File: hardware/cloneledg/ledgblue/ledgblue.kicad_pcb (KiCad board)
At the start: 2 copper layers, 62.4 x 46.9 mm, 61 parts, among them J1 USB_OTG, P1 DEBUG, P2 DEBUG, P3 YL035MY2, P4 YL035MY2_TS_WURTH, SW1 WURTH 436353045816, SW2 SW-PB, U1 LD39020_3.0V, U2 STMPS2151TTR, U3 ST31G480, U4 STM32L476RCT6, U5 AMS_AS3921, U6 STNS01PUR, U7 SPBTLE-RF, U8 STLA02PUR, Y1 8 MHz

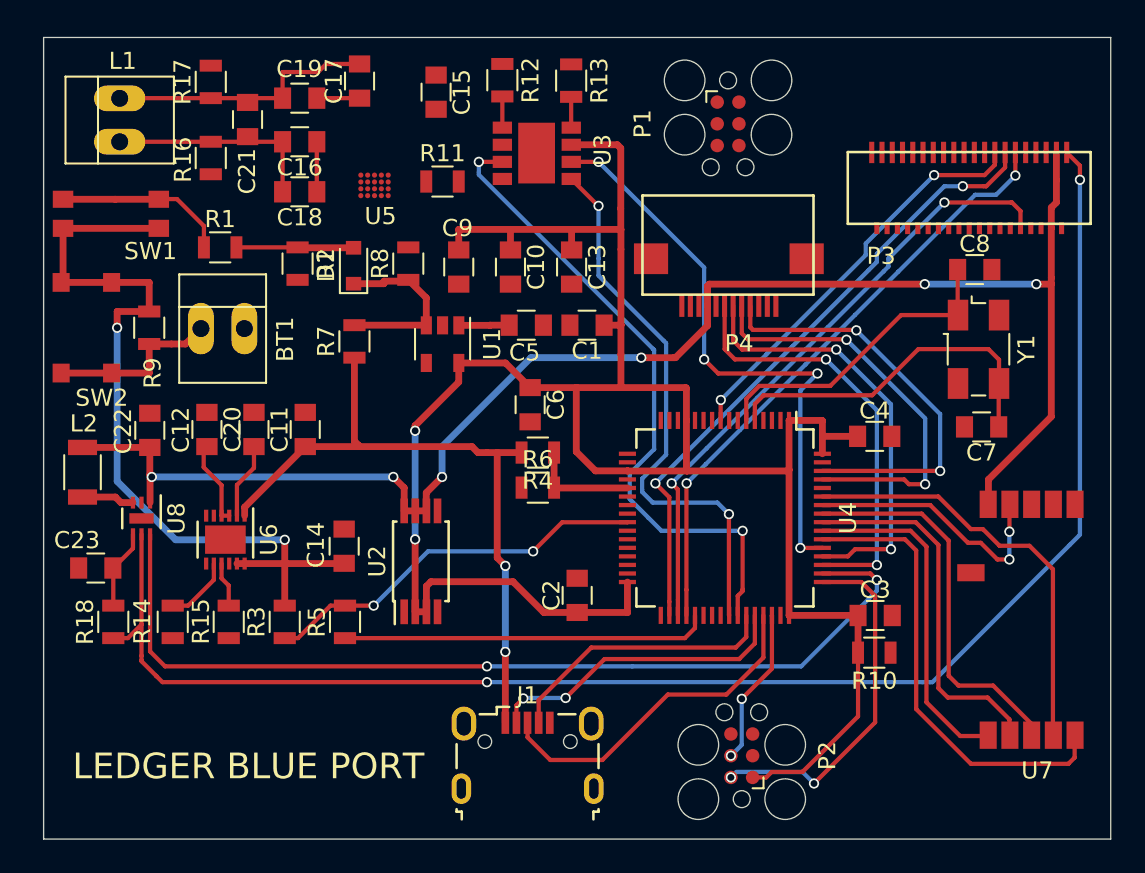
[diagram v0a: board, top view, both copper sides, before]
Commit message: Ledger Blue port finished
Everything is connected!
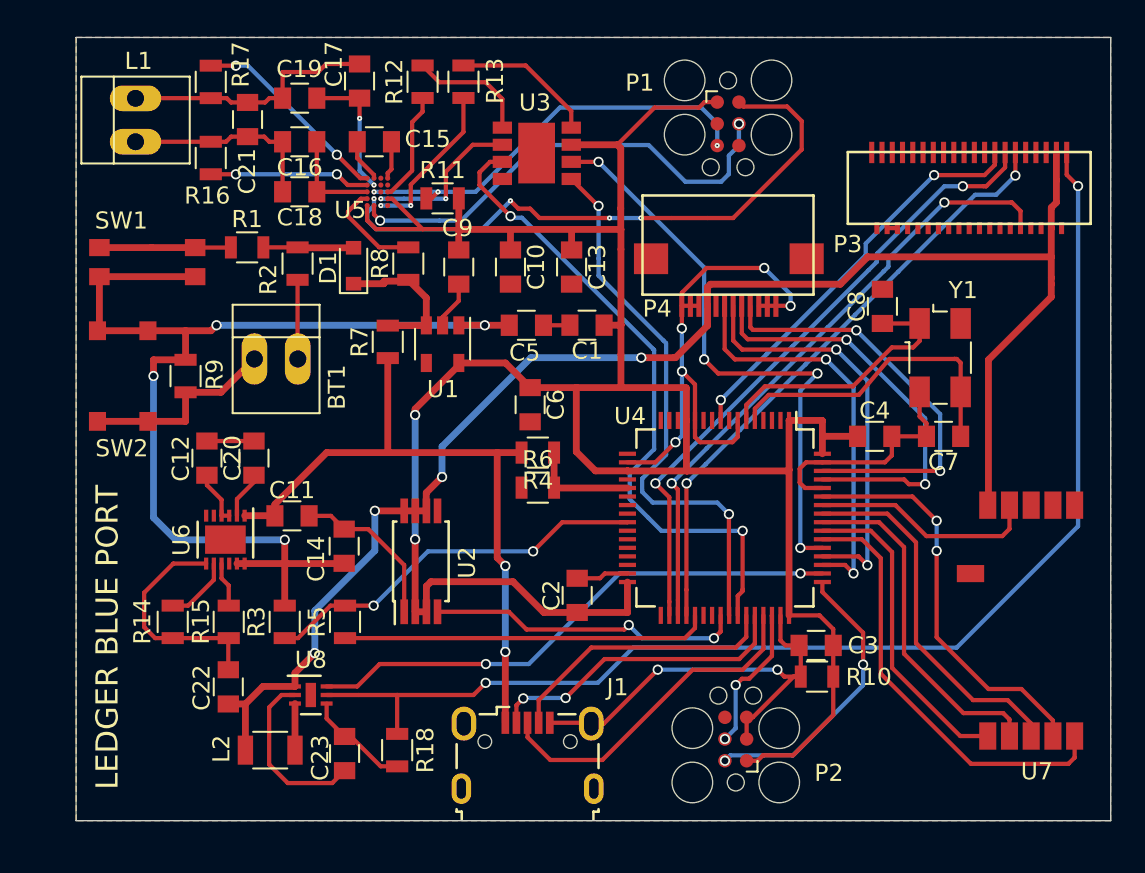
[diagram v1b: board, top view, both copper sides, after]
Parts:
- moved L2 19.6 mm to (39.0, 179.3), turned to 180 degrees
- moved R18 18.2 mm to (46.5, 179.3), turned to 270 degrees
- moved C23 18.2 mm to (43.4, 179.5), turned to 270 degrees
- moved C22 15.7 mm to (36.6, 175.6)
- moved U8 14.3 mm to (41.4, 176.1), turned to 0 degrees
- moved R13 6.30 mm to (50.4, 140.2), turned to 90 degrees
- moved C8 5.81 mm to (74.8, 153.3), turned to 90 degrees
- moved C11 5.11 mm to (40.3, 165.6), turned to 0 degrees
- moved R12 4.67 mm to (48.0, 140.2), turned to 90 degrees
- moved C15 4.63 mm to (45.1, 143.7), turned to 0 degrees
- moved C3 3.87 mm to (71.0, 173.2), turned to 180 degrees
- moved R10 3.63 mm to (71.0, 175.0), turned to 0 degrees
- moved BT1 3.59 mm to (38.1, 156.4)
- moved R9 3.54 mm to (34.1, 157.4)
- moved SW1 3.54 mm to (28.5, 149.4)
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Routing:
- net NRST: track 0.00 -> 137.4 mm, vias 0 -> 9
- net Net-(P1-Pad2): track 0.00 -> 35.6 mm, vias 0 -> 4
- net Net-(P1-Pad4): track 0.00 -> 27.5 mm, vias 0 -> 2
- net Net-(P1-Pad5): track 0.00 -> 24.6 mm, vias 0 -> 3
- net Backlight_PWM: track 55.5 -> 31.7 mm
- net LED_A: track 91.1 -> 72.4 mm
- net AUX_PWR_enable: track 0.00 -> 18.5 mm, vias 0 -> 2
- net MAIN_POWER: track 133.7 -> 148.1 mm
- net +BATT: track 51.8 -> 65.7 mm, vias 2 -> 4
- net Net-(R17-Pad2): track 0.00 -> 11.9 mm, vias 0 -> 2
- net Net-(R16-Pad2): track 0.00 -> 9.41 mm, vias 0 -> 2
- net Net-(R13-Pad1): track 0.00 -> 9.32 mm, vias 0 -> 2
- net Net-(R13-Pad2): track 1.80 -> 8.39 mm
- net Net-(R12-Pad1): track 0.00 -> 6.45 mm
- net Net-(C17-Pad1): track 2.50 -> 7.93 mm, vias 0 -> 2
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- added copper zone on B.Cu, net NRST
- added copper zone on F.Cu, net NRST
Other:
- board size 62.4 x 46.9 mm -> 60.5 x 45.8 mm
- net class Default: clearance 0.1 -> 0.05
- net class MiniVia added: clearance 0.05, trace_width 0.2, via_dia 0.3, via_drill 0.15
- rule trace_clearance: 0.1 -> 0.05
- rule via_min_drill: 0.3 -> 0.1
- rule via_min_size: 0.4 -> 0.3
